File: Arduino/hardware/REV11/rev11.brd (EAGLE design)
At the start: 79 x 79 mm, 31 parts, among them IC2 ATMEGA168-AU, Q1 32768Hz

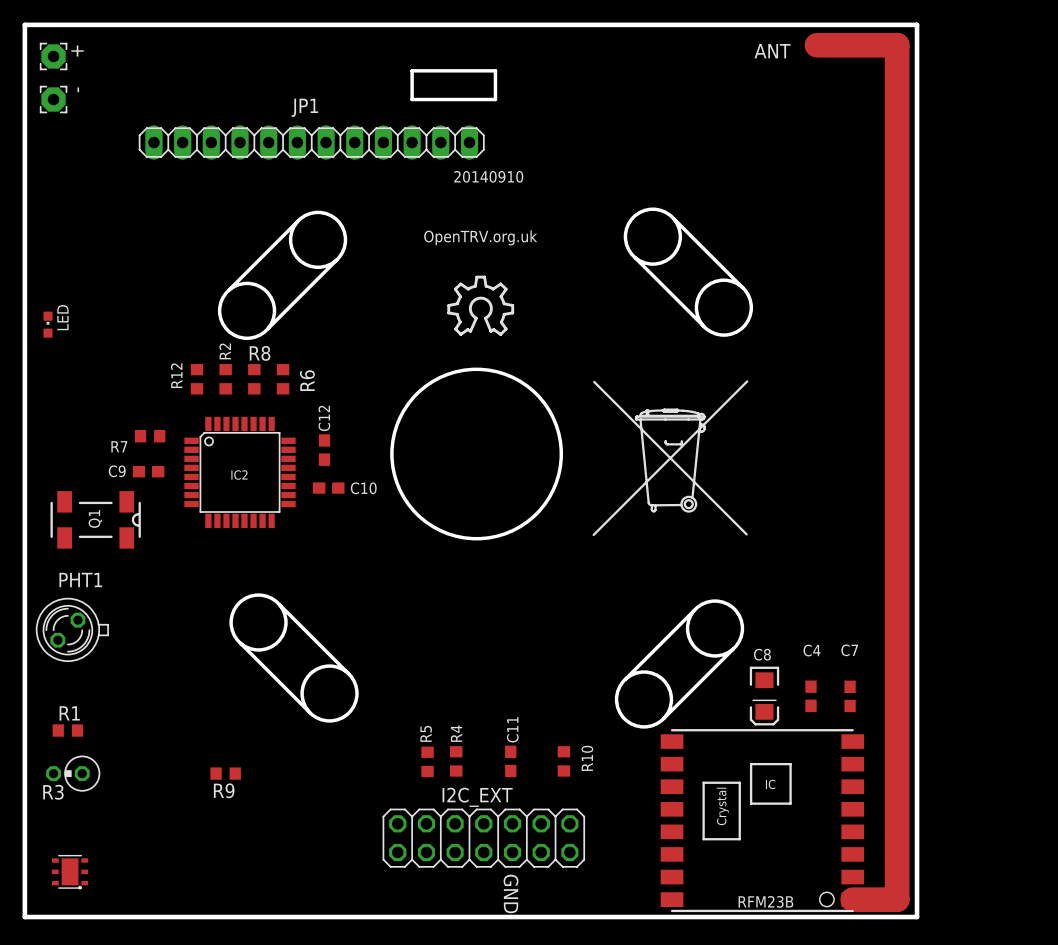
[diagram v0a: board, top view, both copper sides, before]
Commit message: updates to both rev10 and rev11
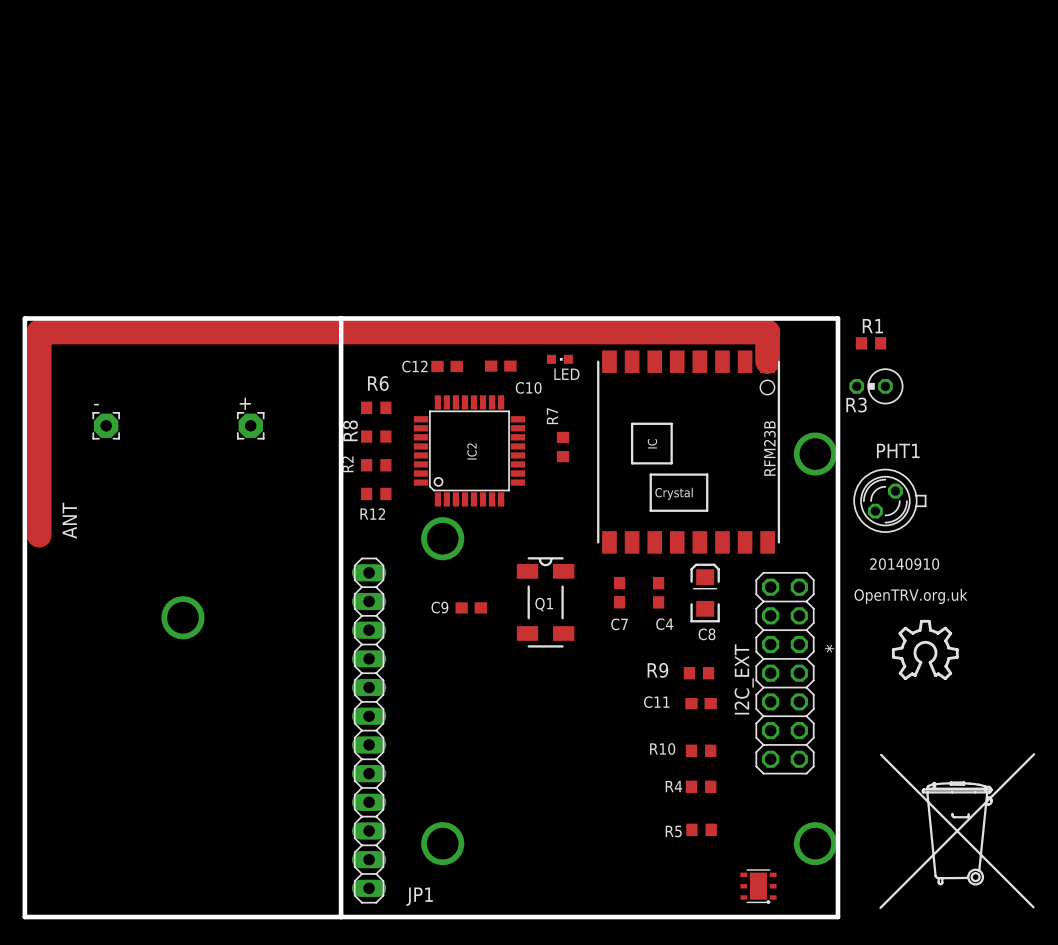
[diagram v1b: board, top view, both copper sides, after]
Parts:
- moved ANT 81.5 mm to (1.27, 34.9), turned to 0 degrees
- moved R1 79.0 mm to (74.9, 50.8)
- moved R3 79.0 mm to (74.9, 47.0)
- moved PHT1 73.3 mm to (76.2, 36.8)
- moved U$4 61.0 mm to (65.0, 2.73)
- moved JP1 52.3 mm to (30.5, 16.5), turned to 270 degrees
- moved U$1 49.8 mm to (76.9, 21.1)
- moved LED 45.4 mm to (47.4, 49.4), turned to 270 degrees
- moved R9 42.8 mm to (59.7, 21.6)
- moved U$2 41.7 mm to (82.4, 4.86)
- moved Q1 40.5 mm to (46.1, 27.9), turned to 270 degrees
- moved + 37.1 mm to (20.0, 43.5), turned to 0 degrees
- moved R7 36.6 mm to (47.7, 41.6), turned to 90 degrees
- moved RFM23B 33.3 mm to (58.8, 41.2), turned to 270 degrees
- moved C9 31.0 mm to (39.5, 27.4)
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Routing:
- net N$31: track 86.7 -> 85.1 mm
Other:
- board size 79 x 79 mm -> 72 x 53 mm
- board text added: "*"
- board text removed: "GND"
